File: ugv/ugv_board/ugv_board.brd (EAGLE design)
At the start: 65 x 56 mm, 36 parts, among them IC1 V7805-1000, U1 DRV8835, U2 MPU-9250, U3 DRV8835, U4 DRV8835, U5 DRV8835

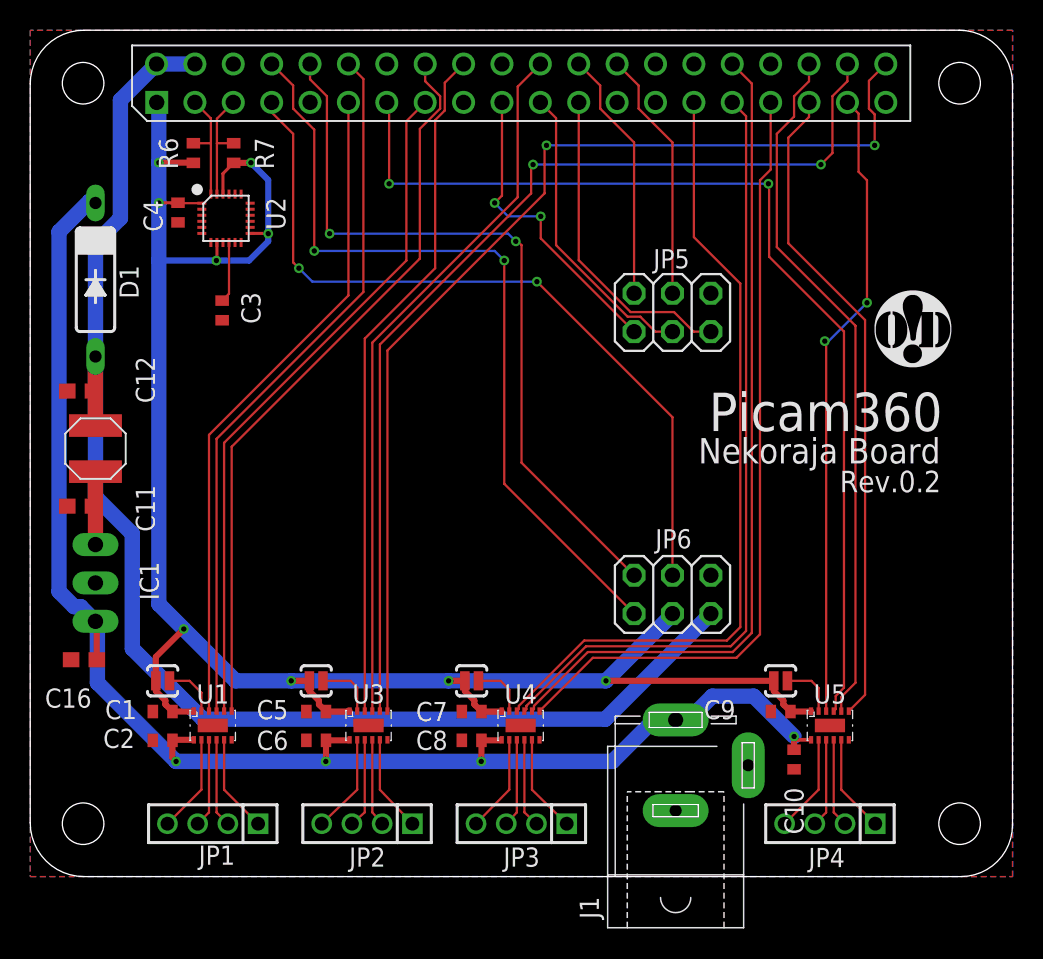
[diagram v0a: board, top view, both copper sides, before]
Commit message: ugv : before v1.0
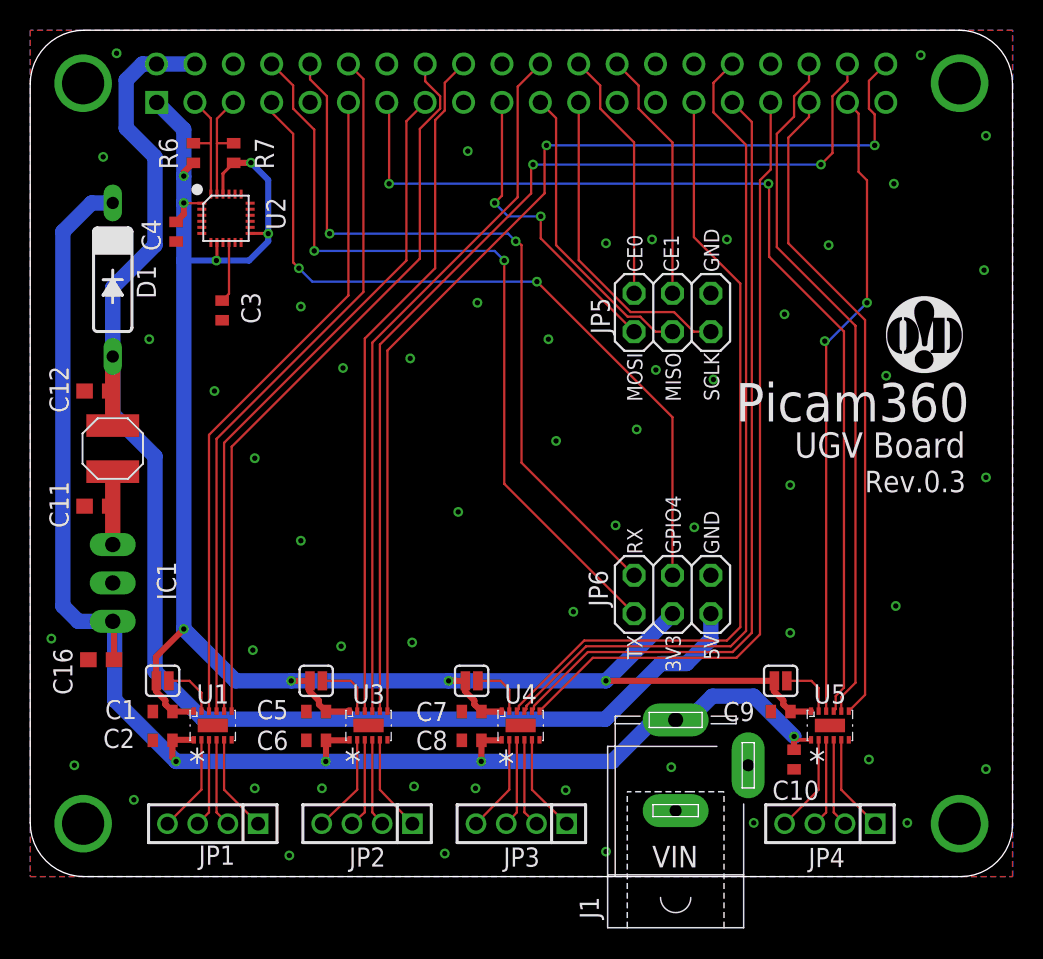
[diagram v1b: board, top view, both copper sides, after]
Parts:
- PCB1: device nekojara_board:RPI3 -> ugv_board:RPI3
- SJ1, SJ2, SJ3, SJ4: value SOLDERJUMPERNO -> SOLDERJUMPERNC; device SparkFun-Retired:SJ_2S-NO -> SparkFun-Retired:SJ_2S
- moved C4 1.28 mm to (9.65, 42.7)
- moved D1 1.14 mm to (5.46, 39.5)
- moved L1 1.14 mm to (5.46, 28.3)
- moved C11 1.14 mm to (4.45, 24.5)
- moved C12 1.14 mm to (4.45, 32.1)
- moved C16 1.14 mm to (4.70, 14.4)
- moved IC1 1.14 mm to (2.92, 19.4)
- moved U$1 0.85 mm to (59.2, 35.8)
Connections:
- net MD3_A2: now also PCB1.P$32; no longer PCB1.P$31
- net MD3_B1: now also PCB1.P$31; no longer PCB1.P$32
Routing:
- net +3V3: track 130.0 -> 126.4 mm
- net MD3_A2: track 52.3 -> 55.9 mm
- net MD3_B1: track 55.0 -> 52.5 mm
- net +5V: track 93.9 -> 96.1 mm
- net +12V: track 98.9 -> 100.7 mm
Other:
- board text added: "*"
- board text added: "3V3"
- board text added: "5V"
- board text added: "CE0"
- board text added: "CE1"
- board text added: "GND"
- board text added: "GPIO4"
- board text added: "MISO"
- board text added: "MOSI"
- board text added: "RX"
- board text added: "Rev.0.3"
- board text added: "SCLK"
- board text added: "TX"
- board text added: "UGV Board"
- board text added: "VIN"
- board text removed: "Nekoraja Board"
- board text removed: "Rev.0.2"
